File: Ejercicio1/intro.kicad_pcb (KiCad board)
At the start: 2 copper layers, 21.6 x 16.5 mm, 6 parts, among them K1 CONN_3

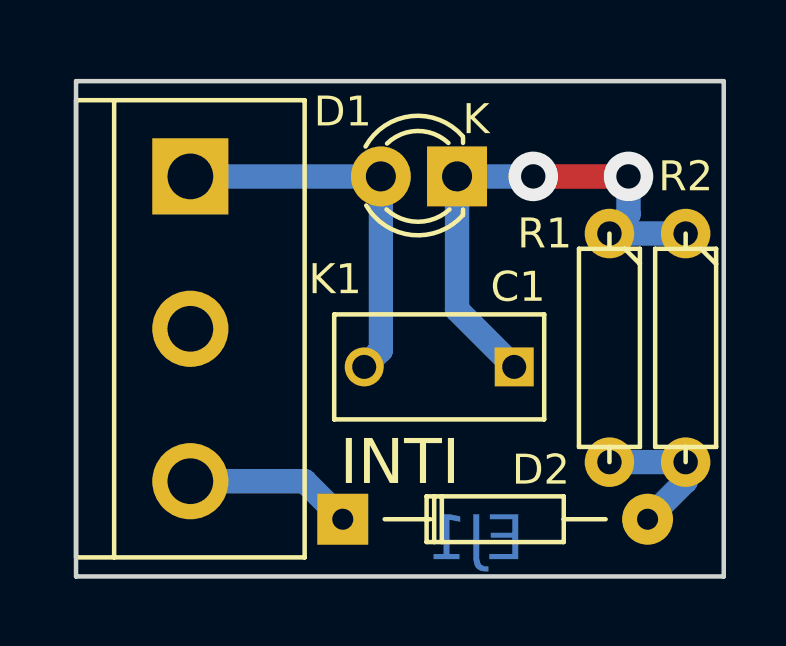
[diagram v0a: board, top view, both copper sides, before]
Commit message: Versión nueva del Ejercicio 1 de Kicad Tour.
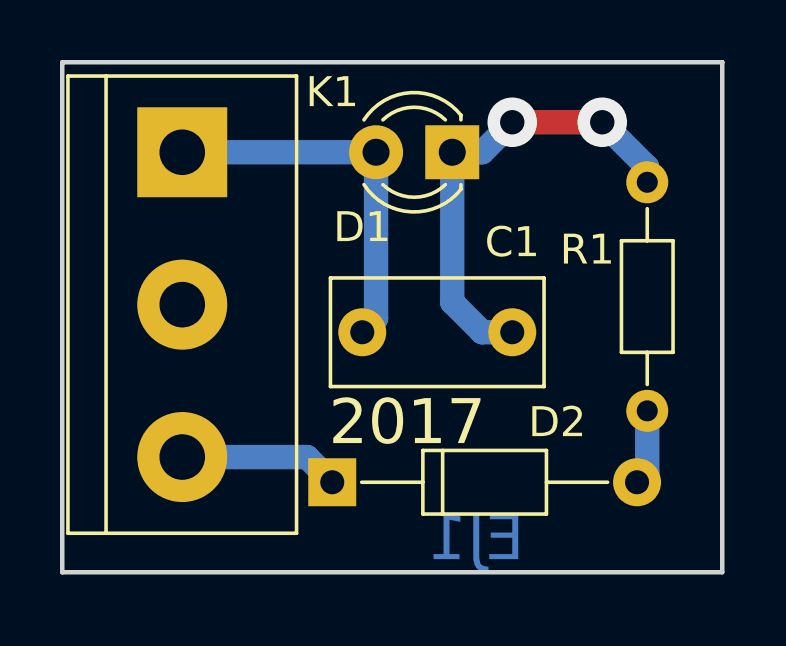
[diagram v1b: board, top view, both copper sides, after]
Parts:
- removed R2: 100K, footprints_ej1:R3-LARGE_PADS
- C1: footprint footprints_ej1:C_Rect_L7_W3.5_P5 -> Capacitors_THT:C_Rect_L7.0mm_W3.5mm_P5.00mm
- D1: footprint footprints_ej1:LED-3MM -> LEDs:LED_D3.0mm
- D2: footprint footprints_ej1:Diode_DO-35_SOD27_Horizontal_RM10 -> Diodes_THT:D_DO-35_SOD27_P10.16mm_Horizontal
- K1: footprint footprints_ej1:bornier3 -> Connectors:bornier3
- R1: footprint footprints_ej1:R3-LARGE_PADS -> Resistors_THT:R_Axial_DIN0204_L3.6mm_D1.6mm_P7.62mm_Horizontal
- moved K1 5.89 mm to (128.0, 90.0)
- moved R1 5.66 mm to (143.5, 91.0)
- moved D2 1.28 mm to (133.0, 101.0)
- moved C1 1.16 mm to (139.0, 96.0)
- moved D1 0.82 mm to (137.0, 90.0)
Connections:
- K1 pad 2: (no net) -> Net-(K1-Pad2)
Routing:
- net Net-(D2-Pad2): track 4.97 -> 2.52 mm
- net Net-(C1-Pad1): track 17.6 -> 15.4 mm
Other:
- board size 21.6 x 16.5 mm -> 22 x 17 mm
- net class Default: clearance 0.889 -> 0.9
- rule trace_clearance: 0.889 -> 0.9
- board text added: "2017"
- board text removed: "INTI"
